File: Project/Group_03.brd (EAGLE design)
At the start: 100 x 80 mm, 29 parts, among them J1 POWER_JACKPTH_LOCK, U1 +12v, U3 TCA9546APW, U4 TMUX1208RSV

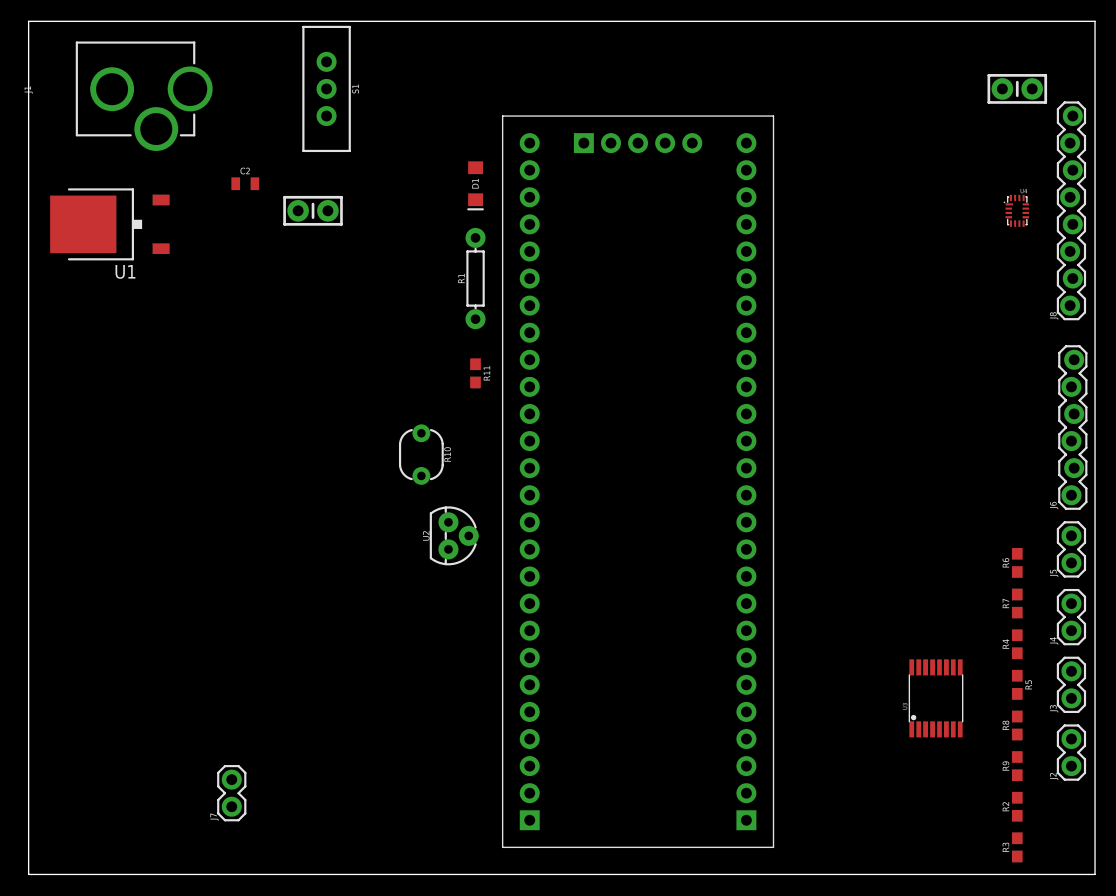
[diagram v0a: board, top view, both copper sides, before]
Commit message: Parts placement (size 73.66x71.12)
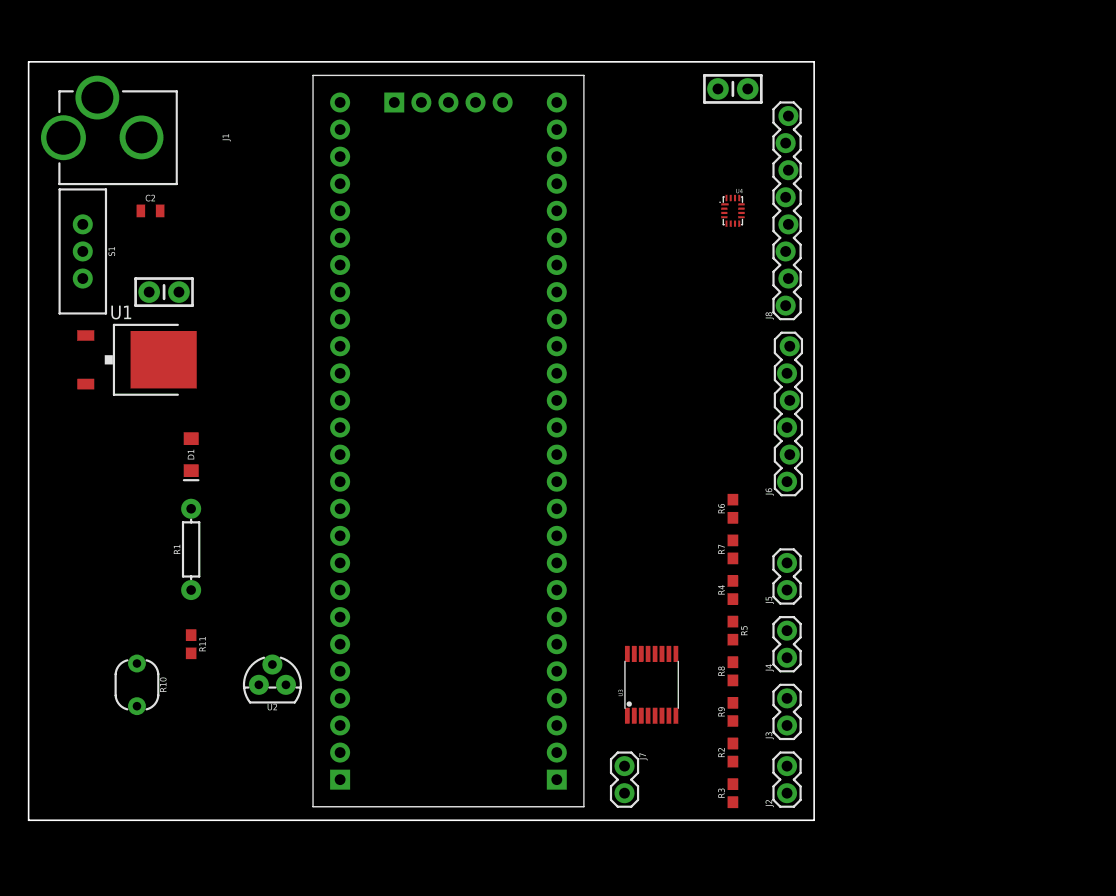
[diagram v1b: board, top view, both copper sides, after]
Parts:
- moved J7 37.0 mm to (55.9, 10.2), turned to 270 degrees
- moved D1 36.8 mm to (15.2, 39.4)
- moved R1 36.8 mm to (15.2, 30.5)
- moved R11 36.8 mm to (15.2, 21.6)
- moved R10 34.3 mm to (10.2, 17.8)
- moved S1 27.5 mm to (5.08, 58.4)
- moved R2 27.1 mm to (66.0, 11.4)
- moved R3 27.1 mm to (66.0, 7.62)
- moved R4 27.1 mm to (66.0, 26.7)
- moved R5 27.1 mm to (66.0, 22.9)
- moved R6 27.1 mm to (66.0, 34.3)
- moved R7 27.1 mm to (66.0, 30.5)
- moved R8 27.1 mm to (66.0, 19.1)
- moved R9 27.1 mm to (66.0, 15.2)
- moved J2 26.8 mm to (71.1, 7.62)
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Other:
- board size 100 x 80 mm -> 73.7 x 71.1 mm
